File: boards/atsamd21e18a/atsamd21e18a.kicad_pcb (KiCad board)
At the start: 4 copper layers, 17.8 x 38.1 mm, 25 parts, among them J1 USB_B_Micro, J2 A, J3 B, J4 SWD_1.27, SW1 RESET, U1 AP7361C_SOT-89-5, U2 ATSAMD21E, Y1 ABS07-32.768KHZ

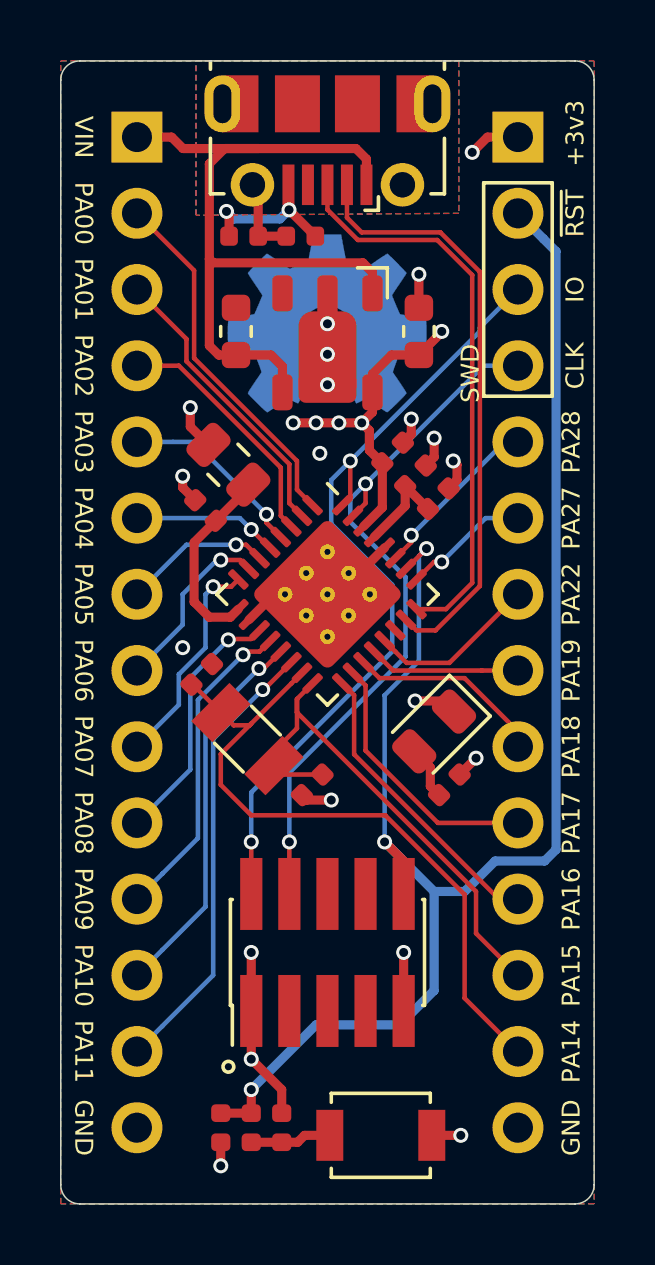
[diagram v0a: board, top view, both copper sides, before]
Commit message: Version 2020-04 looks good. Next: panelize.
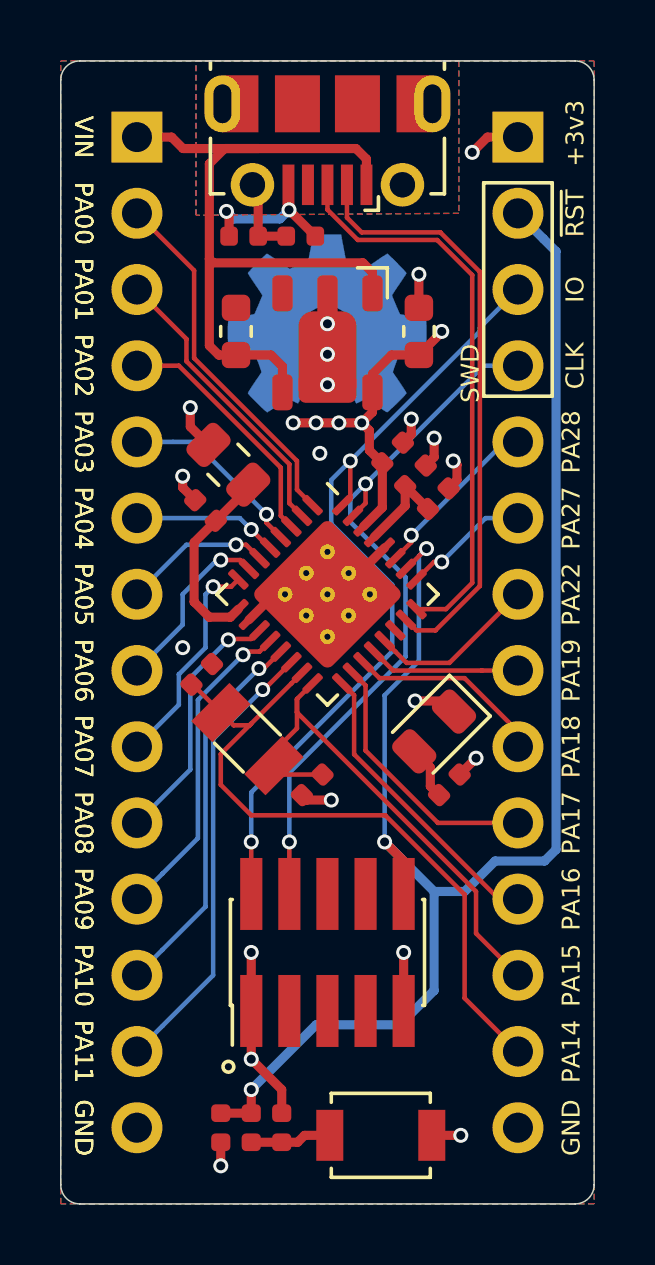
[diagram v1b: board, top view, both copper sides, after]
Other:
- board text added: "atsamd21e18a 2020-04 fourside.io"
- board text removed: "atsamd21e18a 2020-03 fourside.io"
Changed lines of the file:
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@@
   (general
     (thickness 1.6)
-    (drawings 43)
+    (drawings 57)
     (tracks 314)
     (zones 0)
@@
   )
   (setup
-    (last_trace_width 0.3048)
+    (last_trace_width 0.1524)
     (user_trace_width 0.1524)
     (user_trace_width 0.2032)
@@
     )
   )
+  (gr_text PA06 (at 27.432 43.18 270) (layer F.SilkS)
+    (effects (font (size 0.6 0.6) (thickness 0.1)))
+  )
+  (gr_text PA11 (at 27.432 55.88 270) (layer F.SilkS)
+    (effects (font (size 0.6 0.6) (thickness 0.1)))
+  )
+  (gr_text PA01 (at 27.432 30.48 270) (layer F.SilkS)
+    (effects (font (size 0.6 0.6) (thickness 0.1)))
+  )
+  (gr_text PA02 (at 27.432 33.02 270) (layer F.SilkS)
+    (effects (font (size 0.6 0.6) (thickness 0.1)))
+  )
+  (gr_text PA00 (at 27.432 27.94 270) (layer F.SilkS)
+    (effects (font (size 0.6 0.6) (thickness 0.1)))
+  )
+  (gr_text PA10 (at 27.432 53.34 270) (layer F.SilkS)
+    (effects (font (size 0.6 0.6) (thickness 0.1)))
+  )
+  (gr_text PA04 (at 27.432 38.1 270) (layer F.SilkS)
+    (effects (font (size 0.6 0.6) (thickness 0.1)))
+  )
+  (gr_text PA05 (at 27.432 40.64 270) (layer F.SilkS)
+    (effects (font (size 0.6 0.6) (thickness 0.1)))
+  )
+  (gr_text VIN (at 27.432 25.4 270) (layer F.SilkS)
+    (effects (font (size 0.6 0.6) (thickness 0.1)))
+  )
+  (gr_text PA07 (at 27.432 45.72 270) (layer F.SilkS)
+    (effects (font (size 0.6 0.6) (thickness 0.1)))
+  )
+  (gr_text GND (at 27.432 58.42 270) (layer F.SilkS)
+    (effects (font (size 0.6 0.6) (thickness 0.1)))
+  )
+  (gr_text PA03 (at 27.432 35.56 270) (layer F.SilkS)
+    (effects (font (size 0.6 0.6) (thickness 0.1)))
+  )
+  (gr_text PA08 (at 27.432 48.26 270) (layer F.SilkS)
+    (effects (font (size 0.6 0.6) (thickness 0.1)))
+  )
+  (gr_text PA09 (at 27.432 50.8 270) (layer F.SilkS)
+    (effects (font (size 0.6 0.6) (thickness 0.1)))
+  )
   (gr_text SWD (at 40.3225 33.274 90) (layer F.SilkS)
     (effects (font (size 0.6 0.6) (thickness 0.1)))
@@
     (effects (font (size 0.6 0.6) (thickness 0.1)))
   )
-  (gr_text "atsamd21e18a\n2020-03\nfourside.io" (at 40.005 58.928) (layer B.Mask)
+  (gr_text "atsamd21e18a\n2020-04\nfourside.io" (at 40.005 58.928) (layer B.Mask)
     (effects (font (size 0.6 0.6) (thickness 0.1)) (justify left mirror))
   )
@@
   (gr_line (start 43.815 60.96) (end 27.305 60.96) (layer Edge.Cuts) (width 0.05))
   (gr_line (start 27.305 22.86) (end 43.815 22.86) (layer Edge.Cuts) (width 0.05))
-  (via (at 32.1945 27.8765) (size 0.5) (drill 0.3) (layers F.Cu B.Cu) (net 2))
   (via (at 40.386 25.908) (size 0.5) (drill 0.3) (layers F.Cu B.Cu) (net 1))
   (segment (start 41.91 25.4) (end 40.894 25.4) (width 0.3048) (layer F.Cu) (net 1))
@@
   (via (at 33.02 52.577996) (size 0.5) (drill 0.3) (layers F.Cu B.Cu) (net 1))
   (segment (start 33.02 54.528) (end 33.02 52.577996) (width 0.3048) (layer F.Cu) (net 1))
+  (via (at 32.1945 27.8765) (size 0.5) (drill 0.3) (layers F.Cu B.Cu) (net 2))
   (via (at 35.56 33.655) (size 0.5) (drill 0.3) (layers F.Cu B.Cu) (net 2))
   (via (at 35.56 32.639) (size 0.5) (drill 0.3) (layers F.Cu B.Cu) (net 2))
@@
   (segment (start 32.43338 45.00638) (end 32.961388 45.00638) (width 0.1524) (layer F.Cu) (net 5))
   (segment (start 32.009117 44.582117) (end 32.43338 45.00638) (width 0.1524) (layer F.Cu) (net 5))
-  (segment (start 33.014884 44.952884) (end 34.35792 43.609847) (width 0.1524) (layer F.Cu) (net 5))
   (segment (start 31.076947 43.649947) (end 32.009117 44.582117) (width 0.1524) (layer F.Cu) (net 5))
   (segment (start 31.026053 43.649947) (end 31.076947 43.649947) (width 0.1524) (layer F.Cu) (net 5))
-  (segment (start 33.02 48.006) (end 32.004 46.99) (width 0.1524) (layer F.Cu) (net 5))
-  (segment (start 32.004 46.99) (end 32.004 45.963767) (width 0.1524) (layer F.Cu) (net 5))
-  (segment (start 37.486776 48.006) (end 33.02 48.006) (width 0.1524) (layer F.Cu) (net 5))
   (segment (start 40.132 50.651224) (end 37.486776 48.006) (width 0.1524) (layer F.Cu) (net 5))
   (segment (start 40.132 54.102) (end 40.132 50.651224) (width 0.1524) (layer F.Cu) (net 5))
   (segment (start 41.91 55.88) (end 40.132 54.102) (width 0.1524) (layer F.Cu) (net 5))
+  (segment (start 33.014884 44.952884) (end 34.35792 43.609847) (width 0.1524) (layer F.Cu) (net 5))
   (segment (start 32.004 45.963767) (end 33.014884 44.952884) (width 0.1524) (layer F.Cu) (net 5))
+  (segment (start 32.004 46.99) (end 32.004 45.963767) (width 0.1524) (layer F.Cu) (net 5))
+  (segment (start 33.02 48.006) (end 32.004 46.99) (width 0.1524) (layer F.Cu) (net 5))
+  (segment (start 37.486776 48.006) (end 33.02 48.006) (width 0.1524) (layer F.Cu) (net 5))
   (segment (start 34.544 45.108726) (end 33.791305 45.861421) (width 0.1524) (layer F.Cu) (net 6))
   (segment (start 35.065025 43.609848) (end 34.544 44.130873) (width 0.1524) (layer F.Cu) (net 6))
